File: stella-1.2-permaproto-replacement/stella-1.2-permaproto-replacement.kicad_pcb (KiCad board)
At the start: 2 copper layers, 157 x 51 mm, 15 parts, among them J1 Conn_01x03, J2 Conn_01x04, SW1 RotaryEncoder_Switch, SW2 SW_Push, U1 Eyespi Breakout, U2 RTC, U3 MiniBoost, U4 GPS Breakout, U5 SD Reader

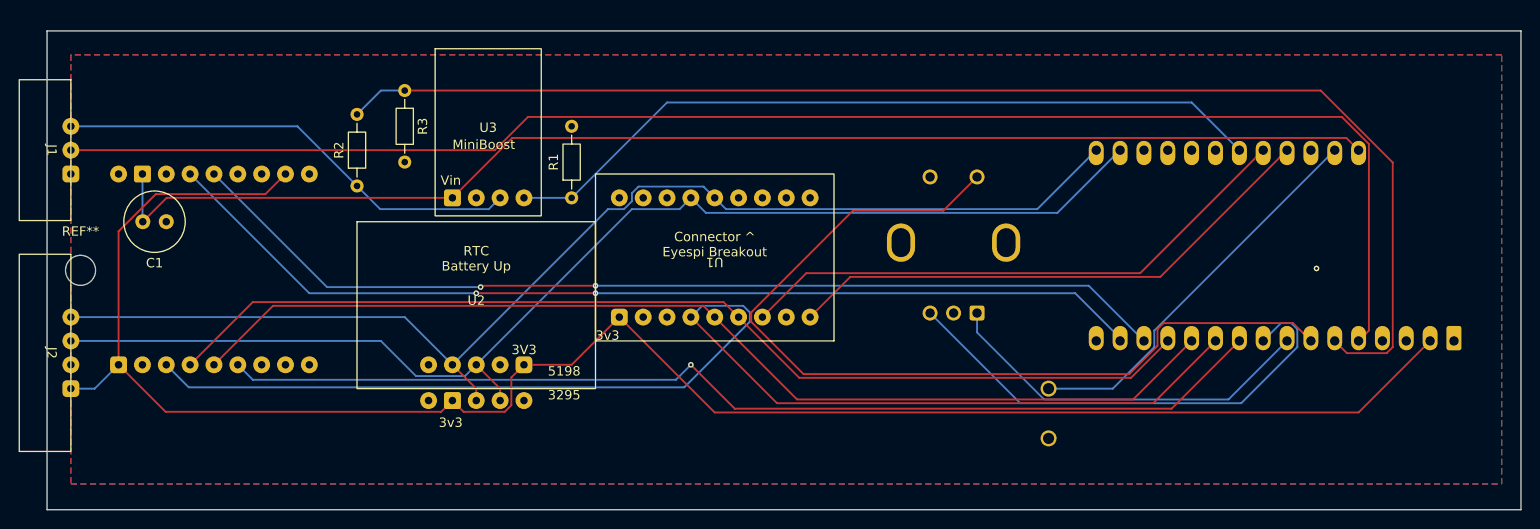
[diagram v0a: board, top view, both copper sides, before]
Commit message: Finalize v0.1.0 of base pcb
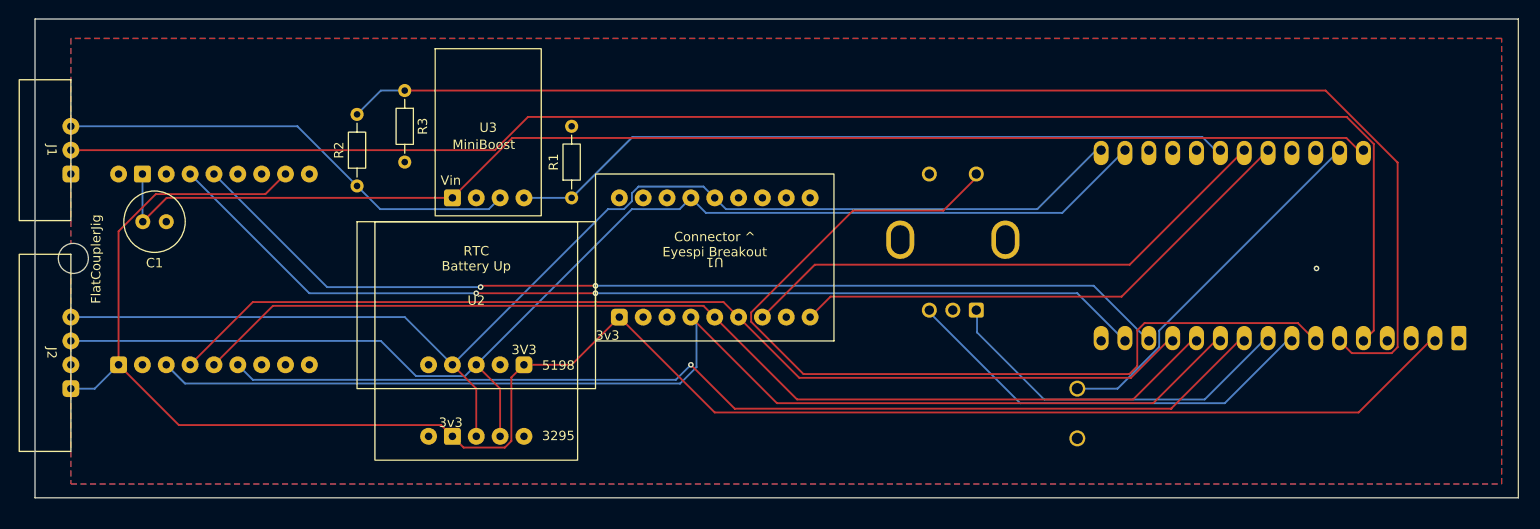
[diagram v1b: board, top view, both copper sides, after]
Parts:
- moved SW2 3.06 mm to (191.0, 114.3)
- moved FlatCouplerJig 1.49 mm to (84.1, 100.4)
- moved A1 0.52 mm to (231.7, 109.2)
- moved SW1 0.32 mm to (180.3, 105.9)
- renumbered REF** to FlatCouplerJig
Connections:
- A1 pad 22: unconnected-(A1-A9/IO33-Pad22) -> Net-(A1-A9/IO33)
- A1 pad 25: Net-(A1-A12/IO13) -> unconnected-(A1-A12/IO13-Pad25)
- R1 pad 1: Net-(A1-A10/IO27) -> Net-(A1-A9/IO33)
- SW1 pad A: Net-(A1-I39/A3) -> Net-(A1-IO36/A4)
- SW1 pad B: Net-(A1-IO36/A4) -> Net-(A1-I39/A3)
- U1 pad 7: Net-(A1-A11/IO12) -> Net-(A1-A10/IO27)
- U1 pad 9: Net-(A1-A12/IO13) -> Net-(A1-A11/IO12)
- U3 pad 4: Net-(A1-A10/IO27) -> Net-(A1-A9/IO33)
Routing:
- net Net-(A1-A9/IO33): track 0.00 -> 76.9 mm
- net Net-(A1-A12/IO13): track 58.2 -> 0.00 mm
- net Net-(A1-A10/IO27): track 82.5 -> 58.7 mm
- net Net-(A1-IO36/A4): track 52.2 -> 38.1 mm
- net /SPI_SCK: track 136.5 -> 126.6 mm
- net Net-(A1-A11/IO12): track 60.7 -> 56.1 mm
- net +3V3: track 196.7 -> 201.1 mm
- net /I2C_SCL: track 129.5 -> 133.8 mm
- net Net-(A1-I39/A3): track 40.6 -> 44.7 mm
- net /I2C_SDA: track 128.1 -> 132.0 mm
- net Net-(A1-EN): track 42.0 -> 39.5 mm
- net Net-(A1-DAC2/A0): track 162.4 -> 164.4 mm
- net Net-(A1-I34/A2): track 97.0 -> 98.7 mm
- net Net-(A1-TX/IO17): track 106.3 -> 106.9 mm
- net Net-(A1-IO4/A5): track 112.9 -> 113.5 mm
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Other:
- board size 157 x 51 mm -> 158 x 51 mm
- board text added: "A1 Adafruit 5447 ESP32-S3 Feather, 4MB Flash 2MB PSRAM Long pins through Feather"
- board text added: "Stella-1.2 Base Permaproto Replacement PCB v0.1.0 2026 Layout by Nathan Eloe Should line up with original permaproto component placement"
